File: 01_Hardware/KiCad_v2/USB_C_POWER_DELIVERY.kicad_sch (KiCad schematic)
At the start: 36 parts, among them Q200 SI7615DN-T1-GE3, Q201 SI7615DN-T1-GE3, Q202 DMP6050SSD-13, Q203 IRLML2402TRPBF, U200 CYPD3177-24LQ

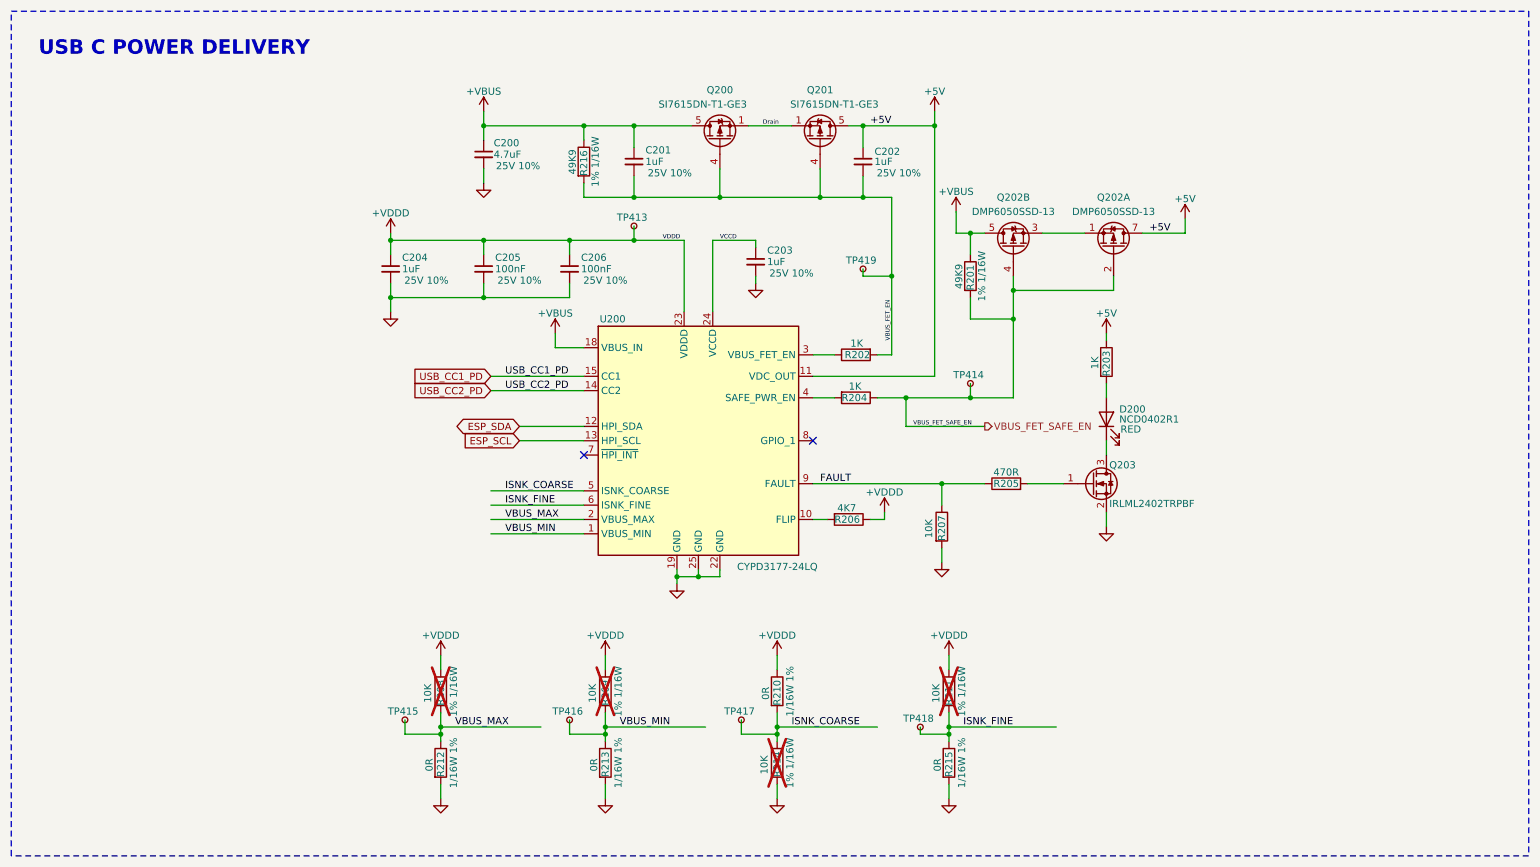
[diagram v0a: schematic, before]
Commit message: Hardware for manufacturing v0.2
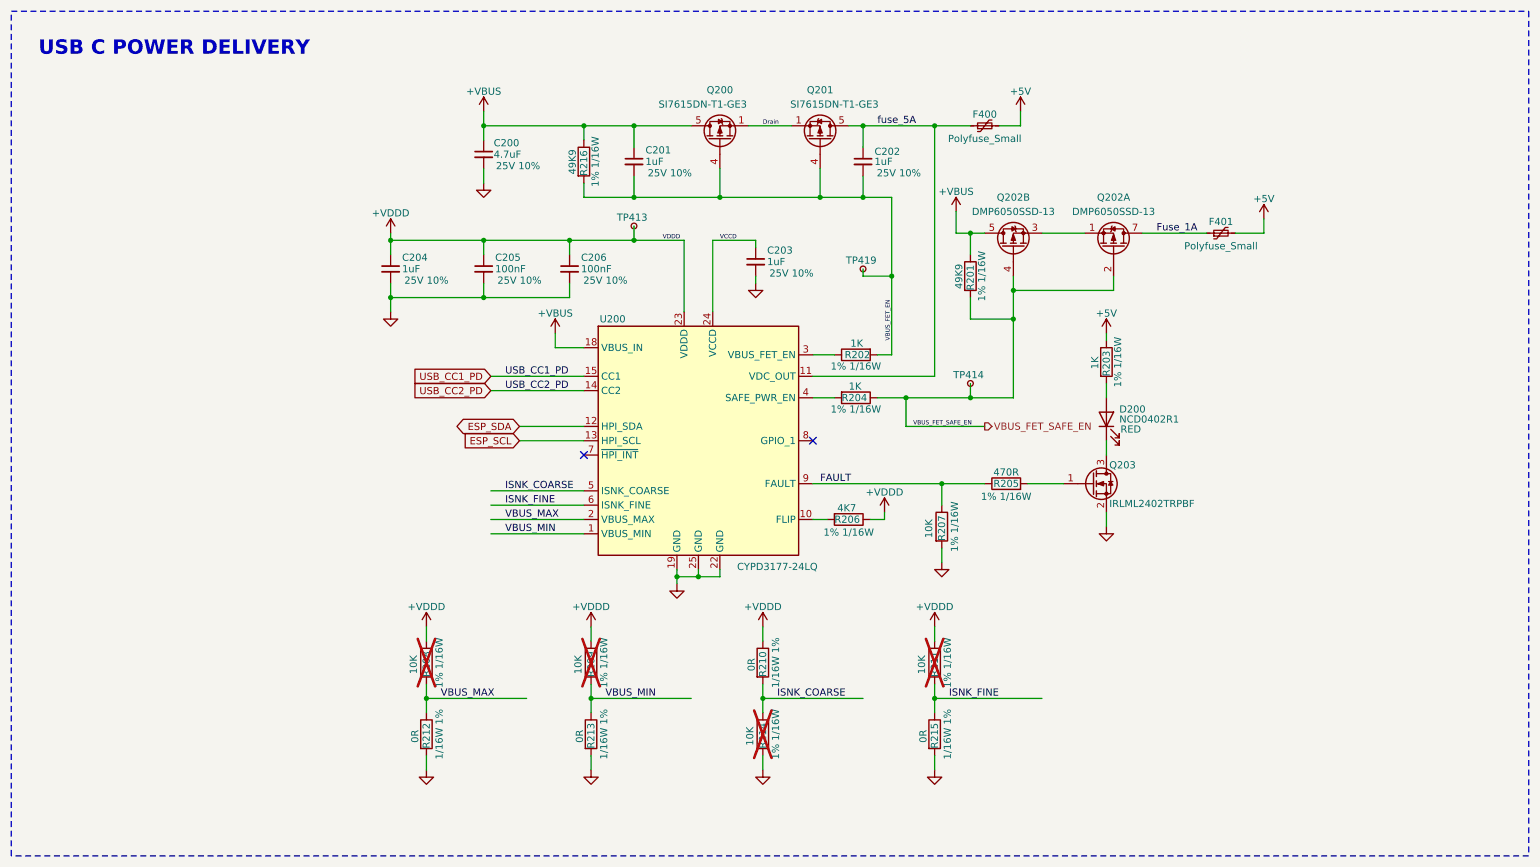
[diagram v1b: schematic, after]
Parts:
- removed TP415, TP416, TP417, TP418: TestPoint_Small, TestPoint:TestPoint_Pad_D1.5mm, symbol Connector:TestPoint_Small
- added F400, F401: Polyfuse_Small, Fuse:Fuse_1210_3225Metric, symbol Device:Polyfuse_Small
- C200: Manufacturer Samsung Electro-Mechanics -> (none); Manufacturer Part Number CL10A475KA8NQNC -> (none)
- TP413, TP414, TP419: footprint TestPoint:TestPoint_Pad_D1.5mm -> TestPoint:TestPoint_Pad_D1.0mm
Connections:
- net +5V: now also F400.2, F401.2; no longer C202.1, Q201.5 (D), Q202.7 (D1), Q202.8 (D1), U200.11 (VDC_OUT)
- new net Fuse_1A: F401.1, Q202.7 (D1), Q202.8 (D1)
- new net fuse_5A: C202.1, F400.1, Q201.5 (D), U200.11 (VDC_OUT)
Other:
- moved on the sheet: R208, R209, R210, R211, R212, R213, R214, R215
